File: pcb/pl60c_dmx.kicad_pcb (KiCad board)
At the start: 2 copper layers, 80 x 54 mm, 39 parts, among them J1 USB-C 16P, J2 XLR-5 female (DMX OUT), J3 DMX pigtail, J4 EXPANSION, J5 UART0, Q1 S8050, SW1 RESET, SW2 BOOT, SW3 USER, U1 ESP32-S3-WROOM-1-N16R8, U2 AMS1117-3.3, U3 SP3485EN, U4 USBLC6-2SC6

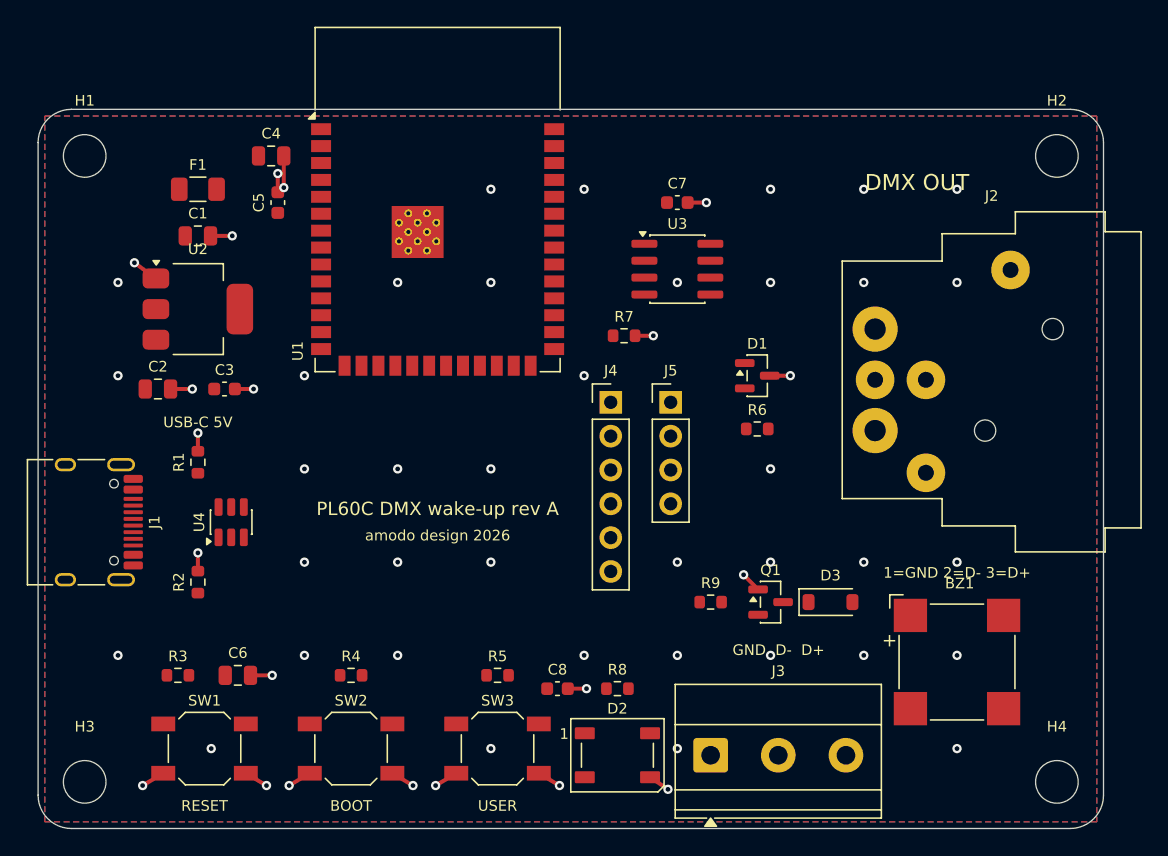
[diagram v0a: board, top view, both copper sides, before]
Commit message: auto: 2026-09-02 13:08:46
Co-Authored-By: Claude Fable 5.1 <noreply@anthropic.com>
Claude-Session: https://claude.ai/code/session_01WsrVZb94LwbHVAmBvsSTfn
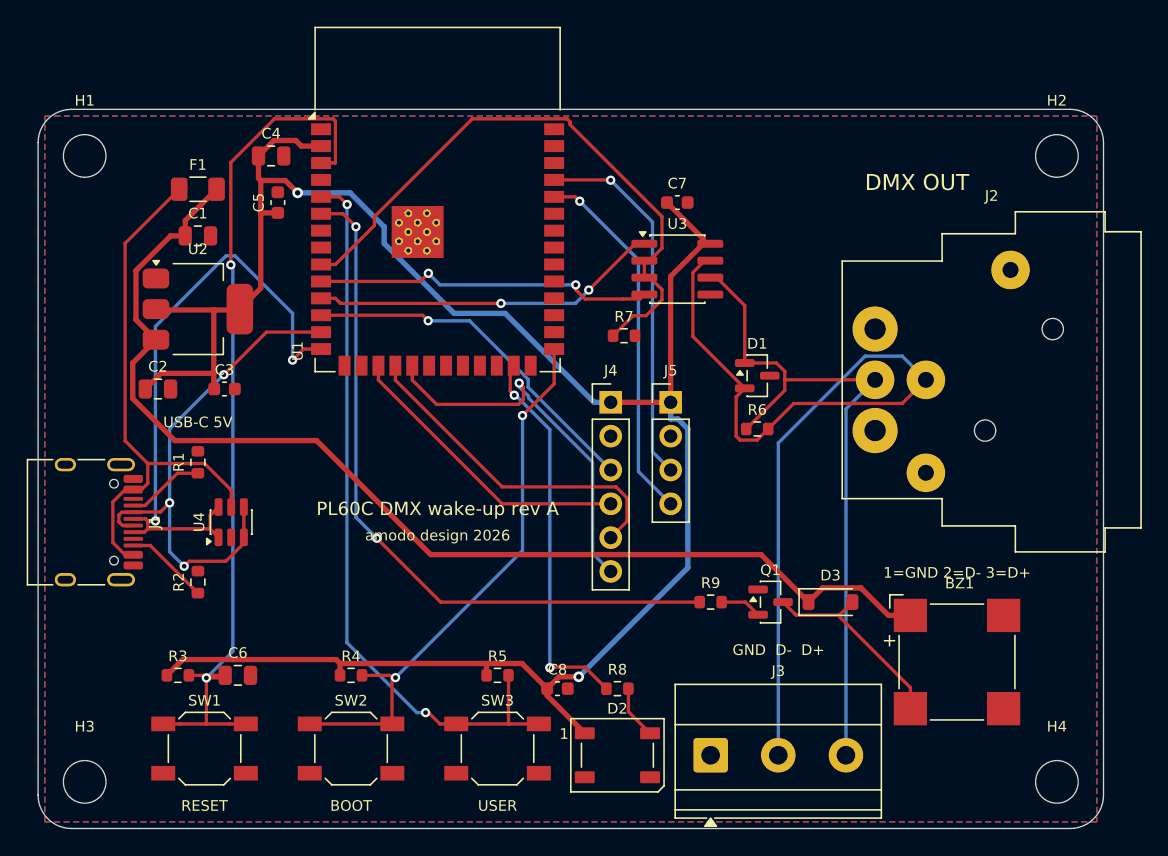
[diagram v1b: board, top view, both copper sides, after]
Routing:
- net +3V3: track 0.00 -> 156.7 mm, vias 0 -> 2
- net +5V: track 0.00 -> 86.2 mm
- net DMX_B: track 0.00 -> 70.1 mm
- net EN: track 0.00 -> 67.0 mm, vias 0 -> 2
- net BTN_USER: track 0.00 -> 55.7 mm, vias 0 -> 2
- net BUZZER: track 0.00 -> 53.3 mm, vias 0 -> 2
- net DMX_A: track 0.00 -> 52.4 mm
- net DMX_DE: track 0.00 -> 46.3 mm
- net USB_D+: track 0.00 -> 45.9 mm, vias 0 -> 2
- net IO0_BOOT: track 0.00 -> 41.9 mm, vias 0 -> 2
- net VBUS: track 0.00 -> 41.0 mm
- net USB_D-: track 0.00 -> 38.9 mm, vias 0 -> 3
- net GND: track 34.5 -> 0.00 mm, vias 59 -> 0
- net LED_DATA: track 0.00 -> 29.0 mm, vias 0 -> 2
- net EXP_IO11: track 0.00 -> 28.7 mm, vias 0 -> 1
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
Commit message: auto: 2026-09-02 13:10:48
Co-Authored-By: Claude Fable 5.1 <noreply@anthropic.com>
Claude-Session: https://claude.ai/code/session_01WsrVZb94LwbHVAmBvsSTfn
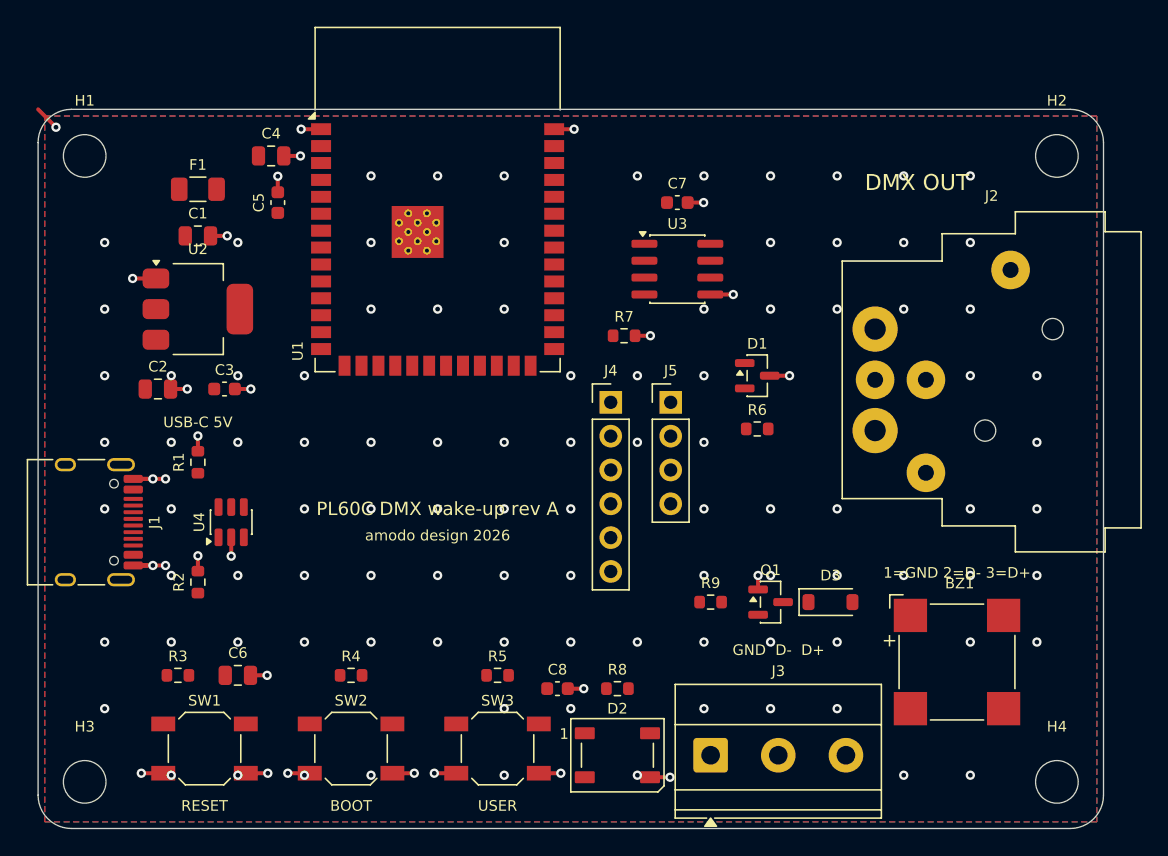
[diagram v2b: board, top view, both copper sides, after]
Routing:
- net +3V3: track 156.7 -> 0.00 mm, vias 2 -> 0
- net +5V: track 86.2 -> 0.00 mm
- net DMX_B: track 70.1 -> 0.00 mm
- net EN: track 67.0 -> 0.00 mm, vias 2 -> 0
- net BTN_USER: track 55.7 -> 0.00 mm, vias 2 -> 0
- net BUZZER: track 53.3 -> 0.00 mm, vias 2 -> 0
- net DMX_A: track 52.4 -> 0.00 mm
- net DMX_DE: track 46.3 -> 0.00 mm
- net USB_D+: track 45.9 -> 0.00 mm, vias 2 -> 0
- net GND: track 0.00 -> 44.8 mm, vias 0 -> 129
- net IO0_BOOT: track 41.9 -> 0.00 mm, vias 2 -> 0
- net VBUS: track 41.0 -> 0.00 mm
- net USB_D-: track 38.9 -> 0.00 mm, vias 3 -> 0
- net LED_DATA: track 29.0 -> 0.00 mm, vias 2 -> 0
- net EXP_IO11: track 28.7 -> 0.00 mm, vias 1 -> 0
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
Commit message: auto: 2026-09-02 13:12:50
Co-Authored-By: Claude Fable 5.1 <noreply@anthropic.com>
Claude-Session: https://claude.ai/code/session_01WsrVZb94LwbHVAmBvsSTfn
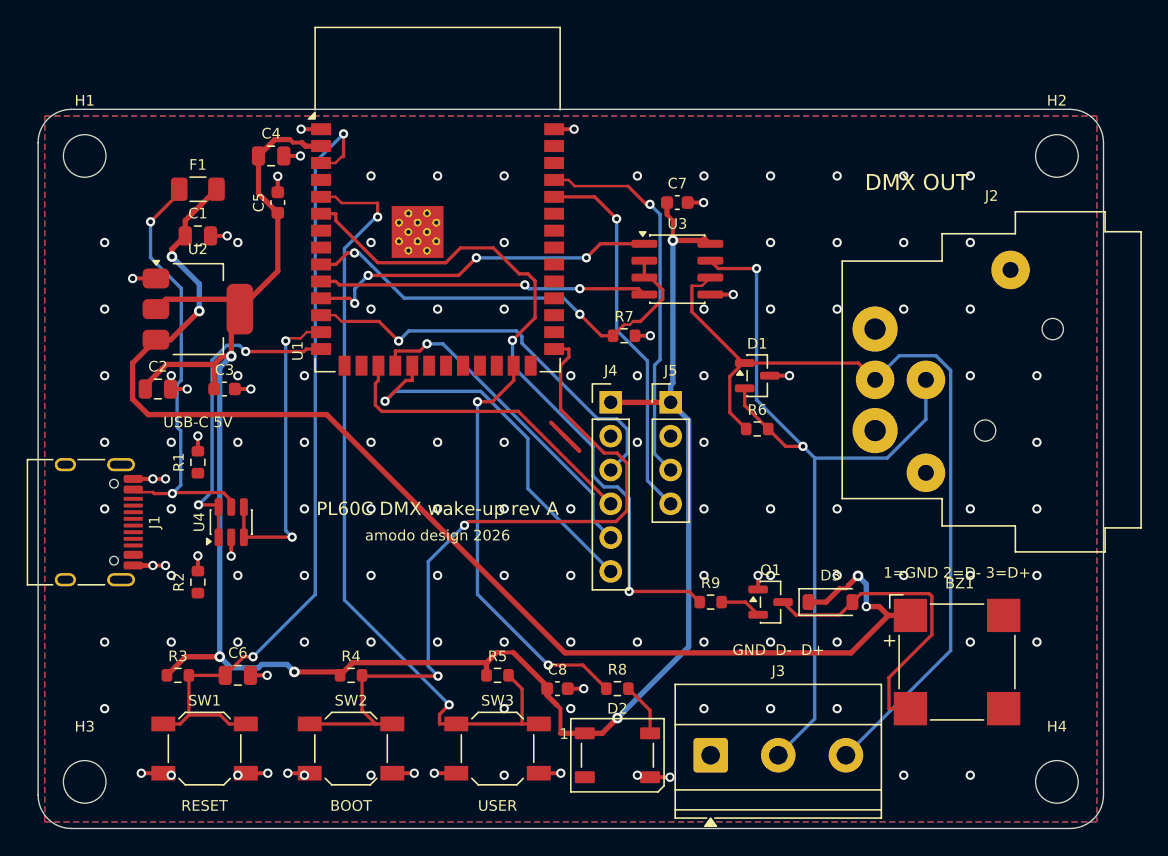
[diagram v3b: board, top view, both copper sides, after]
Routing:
- net +3V3: track 0.00 -> 152.4 mm, vias 0 -> 5
- net +5V: track 0.00 -> 97.2 mm, vias 0 -> 4
- net DMX_A: track 0.00 -> 64.4 mm
- net DMX_B: track 0.00 -> 62.7 mm, vias 0 -> 2
- net EN: track 0.00 -> 60.8 mm, vias 0 -> 2
- net BTN_USER: track 0.00 -> 59.8 mm, vias 0 -> 2
- net IO0_BOOT: track 0.00 -> 57.5 mm, vias 0 -> 2
- net BUZZER: track 0.00 -> 53.2 mm, vias 0 -> 2
- net DMX_DE: track 0.00 -> 33.5 mm, vias 0 -> 2
- net VBUS: track 0.00 -> 33.4 mm, vias 0 -> 2
- net LED_DATA: track 0.00 -> 31.6 mm, vias 0 -> 2
- net EXP_SDA: track 0.00 -> 31.0 mm, vias 0 -> 1
- net TXD0: track 0.00 -> 28.9 mm, vias 0 -> 1
- net EXP_IO11: track 0.00 -> 28.9 mm, vias 0 -> 1
- net RXD0: track 0.00 -> 28.5 mm, vias 0 -> 1
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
